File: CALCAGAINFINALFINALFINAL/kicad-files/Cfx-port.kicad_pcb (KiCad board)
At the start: 4 copper layers, 65 x 99.5 mm, 132 parts, among them J1 Conn_01x11_Socket, J2 USB_C_Receptacle_USB2.0_16P, J3 Micro_SD_Card, J4 Conn_01x02, SW10 SW_SPST, SW100 SW_SPST, SW101 SW_SPST, SW102 SW_SPST, SW49 SW_SPST, SW52 SW_SPST, SW55 SW_SPST, SW56 SW_SPST, SW57 SW_SPST, SW58 SW_SPST, SW59 SW_SPST, SW60 SW_SPST, SW61 SW_SPST, SW62 SW_SPST, SW63 SW_SPST, SW64 SW_SPST, SW65 SW_SPST, SW66 SW_SPST, SW67 SW_SPST, SW68 SW_SPST, SW69 SW_SPST, SW70 SW_SPST, SW71 SW_SPST, SW72 SW_SPST, SW73 SW_SPST, SW74 SW_SPST, SW75 SW_SPST, SW76 SW_SPST, SW77 SW_SPST, SW78 SW_SPST, SW79 SW_SPST, SW80 SW_SPST, SW81 SW_SPST, SW82 SW_SPST, SW83 SW_SPST, SW84 SW_SPST, SW85 SW_SPST, SW86 SW_SPST, SW87 SW_SPST, SW88 SW_SPST, SW89 SW_SPST, SW90 SW_SPST, SW91 SW_SPST, SW92 SW_SPST, SW93 SW_SPST, SW94 SW_SPST, SW95 SW_SPST, SW96 SW_SPST, SW97 SW_SPST, SW98 SW_SPST, SW99 SW_SPST, U5 TP4056-42-ESOP8, U6 TLV61070ADBV, U7 TCA9535DBR, U8 ESP32-S3-WROOM-1

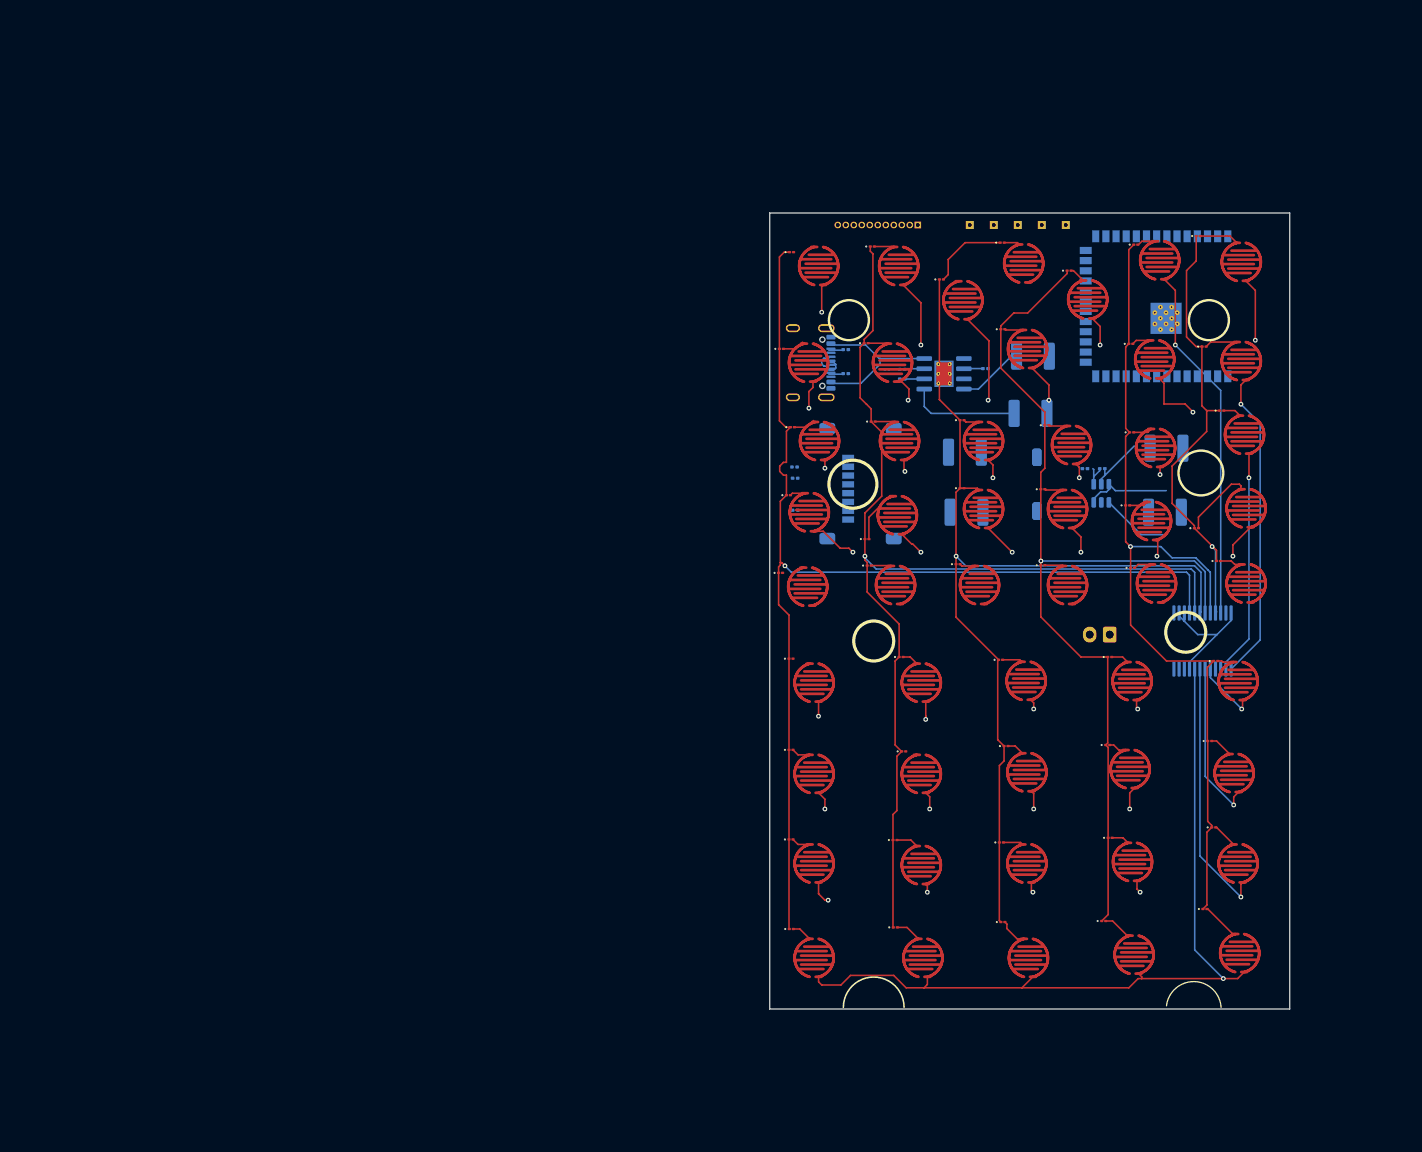
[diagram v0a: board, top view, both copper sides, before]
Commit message: dude this bitch ass project is the fucking boulder of sisyphus omfg ima genuinely kms at this rate if this iteration doesnt work ima genuinely kms like acutal this one is bare esp32 s3 with a diy antenna and crystal like dude what the actual fuck man ima genuinely dei. FINAL FINAL FINAL FINAL ITS GOT THE FUCKING BARE CHIPS FOR DAMN NEAR EVERYTHING DEAR MASS PRODUCED CHINK FACTORY GODS LET THIS THROUGH WITHOUT CAUSING A RUCKUS AND CHARGING LIKE $90 FOR 14 BUCKS OF PARTS AMEN
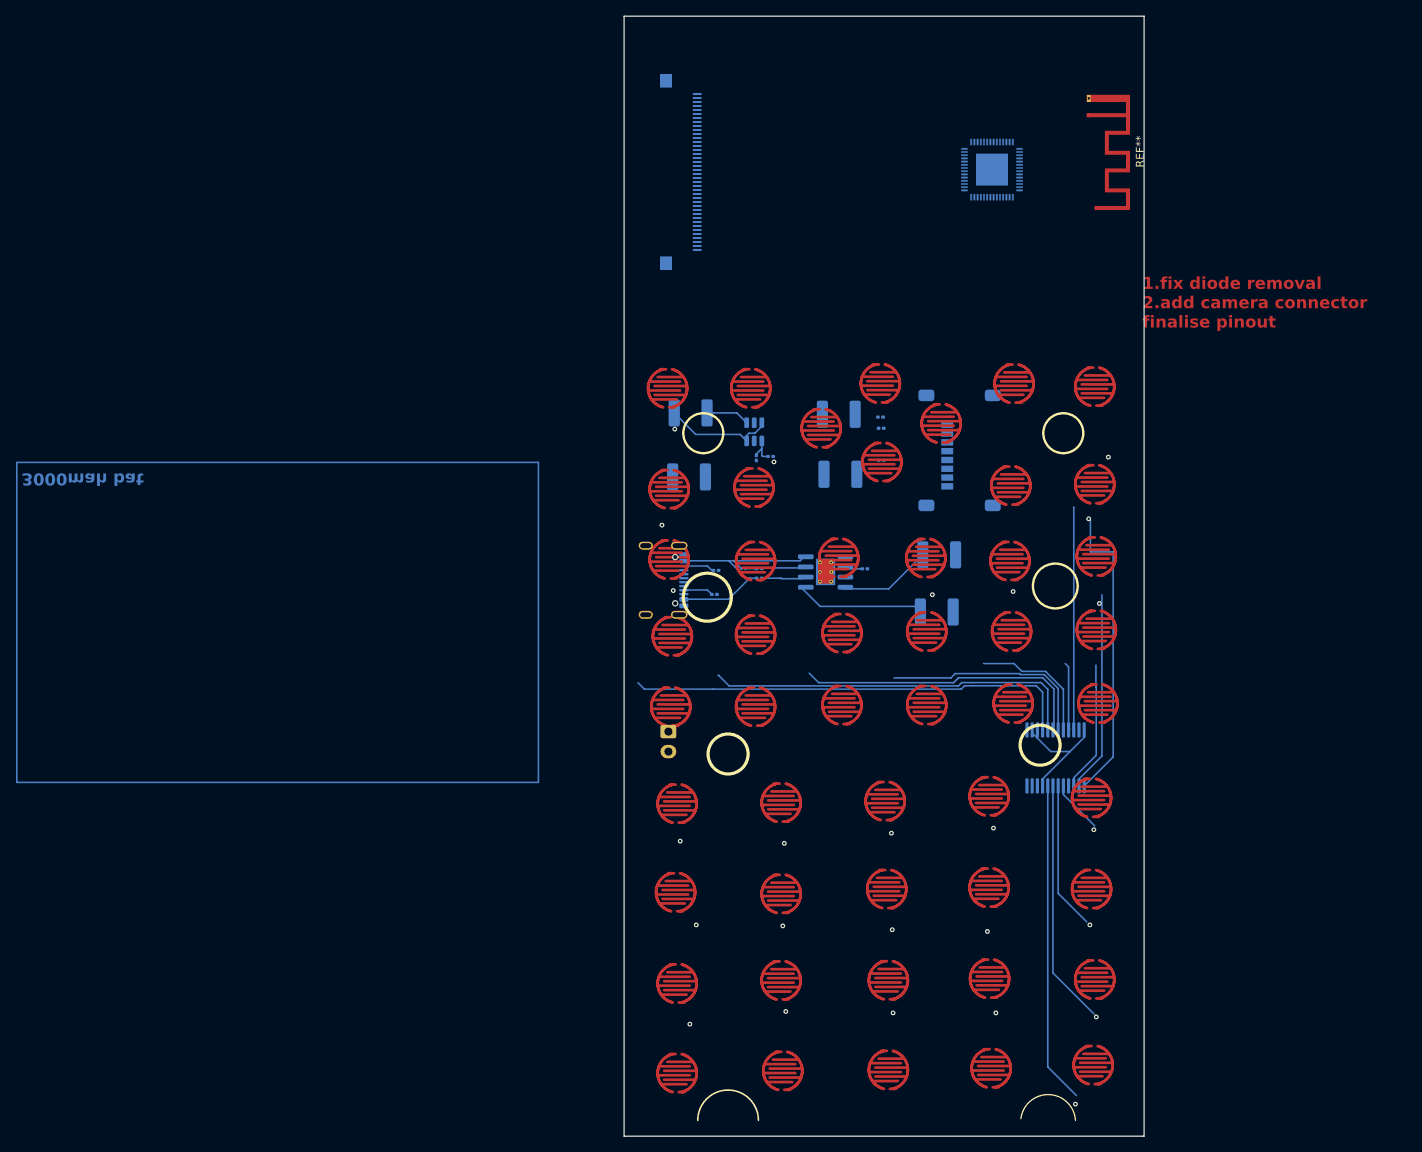
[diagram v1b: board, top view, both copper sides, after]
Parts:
- removed D100, D101, D102, D103, D104, D55, D56, D57, D58, D59, D60, D61, D62, D63, D64, D65, D66, D67, D68, D69, D70, D71, D72, D73, D74, D75, D76, D77, D78, D79, D80, D81, D82, D83, D84, D85, D86, D87, D88, D89, D90, D91, D92, D93, D94, D95, D96, D97, D98, D99: 1N4001, Diode_SMD:D_01005_0402Metric
- removed H1, H2, H3, H4, H5: MountingHole_Pad, TestPoint:TestPoint_THTPad_1.0x1.0mm_Drill0.5mm
- removed J1: Conn_01x11_Socket, Connector_PinSocket_1.00mm:PinSocket_1x11_P1.00mm_Vertical
- removed SW10 (x2): SW_SPST, Button_Switch_SMD:SW_DIP_SPSTx01_Slide_6.7x4.1mm_W6.73mm_P2.54mm_LowProfile_JPin
- removed U8: ESP32-S3-WROOM-1, RF_Module:ESP32-S3-WROOM-1
- added REF**: Texas_SWRA117D_2.4GHz_Right, RF_Antenna:Texas_SWRA117D_2.4GHz_Right, F.Cu at (156.1, 37.4)
- added REF**: Omron_XF2M-4015-1A_1x40-1MP_P0.5mm_Horizontal, Connector_FFC-FPC:Omron_XF2M-4015-1A_1x40-1MP_P0.5mm_Horizontal, B.Cu at (105.1, 44.5)
- added REF1: ESP32-S3R8, ButtonPads:QFN40P700X700X90-57N, B.Cu at (144.0, 44.2)
- moved L2 60.6 mm to (106.3, 74.6), turned to 0 degrees
- moved C6 59.8 mm to (106.1, 82.6), turned to 0 degrees
- moved J4 56.5 mm to (103.5, 114.5), turned to -90 degrees
- moved U6 44.1 mm to (114.3, 77.0), turned to -90 degrees
- moved R14 43.3 mm to (114.5, 80.2), turned to 90 degrees
- moved R13 39.3 mm to (116.3, 80.1), turned to 0 degrees
- moved J2 32.8 mm to (101.8, 95.5)
- moved R8 32.1 mm to (109.3, 97.3)
- moved R9 32.0 mm to (109.5, 94.3)
- moved D15 30.7 mm to (112.9, 94.1)
- moved R10 30.7 mm to (114.9, 94.1)
- moved R11 30.7 mm to (114.9, 95.3)
- moved R12 29.2 mm to (128.1, 94.1)
- moved U5 28.9 mm to (123.2, 94.5)
- moved C4 27.5 mm to (137.4, 92.3)
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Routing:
- net /Keypad Matrix/C4: track 142.0 -> 26.7 mm, vias 1 -> 0
- net /Keypad Matrix/C2: track 162.3 -> 47.4 mm, vias 1 -> 0
- net /Keypad Matrix/C3: track 150.3 -> 37.1 mm, vias 1 -> 0
- net /Keypad Matrix/C1: track 159.8 -> 56.1 mm, vias 1 -> 0
- net /Keypad Matrix/R1: track 126.4 -> 27.8 mm, vias 5 -> 1
- net /Keypad Matrix/C6: track 80.2 -> 8.69 mm, vias 1 -> 0
- net /Keypad Matrix/R6: track 74.6 -> 6.63 mm, vias 5 -> 1
- net GND: track 16.2 -> 76.5 mm, vias 0 -> 3
- net /Keypad Matrix/R9: track 100.4 -> 40.2 mm
- net /Keypad Matrix/R4: track 71.6 -> 16.3 mm, vias 6 -> 0
- net /Keypad Matrix/R2: track 125.8 -> 93.7 mm, vias 6 -> 2
- net /Keypad Matrix/R7: track 81.4 -> 67.6 mm
- net /Keypad Matrix/R3: track 93.6 -> 82.7 mm, vias 6 -> 4
- net /Keypad Matrix/R8: track 94.7 -> 85.9 mm
- net /power-ic/VBAT_SW: track 18.8 -> 25.8 mm
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- added copper zone on In2.Cu, net GND
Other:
- board size 65 x 99.5 mm -> 65 x 140 mm
- board text added: "1.fix diode removal 2.add camera connector finalise pinout"
- board text added: "3000mah bat"
